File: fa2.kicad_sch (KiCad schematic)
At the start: 7 parts, among them U1 4081, U10 4071, U18 4069, U27 4069, U46 4071, U48 4081, U6 4081

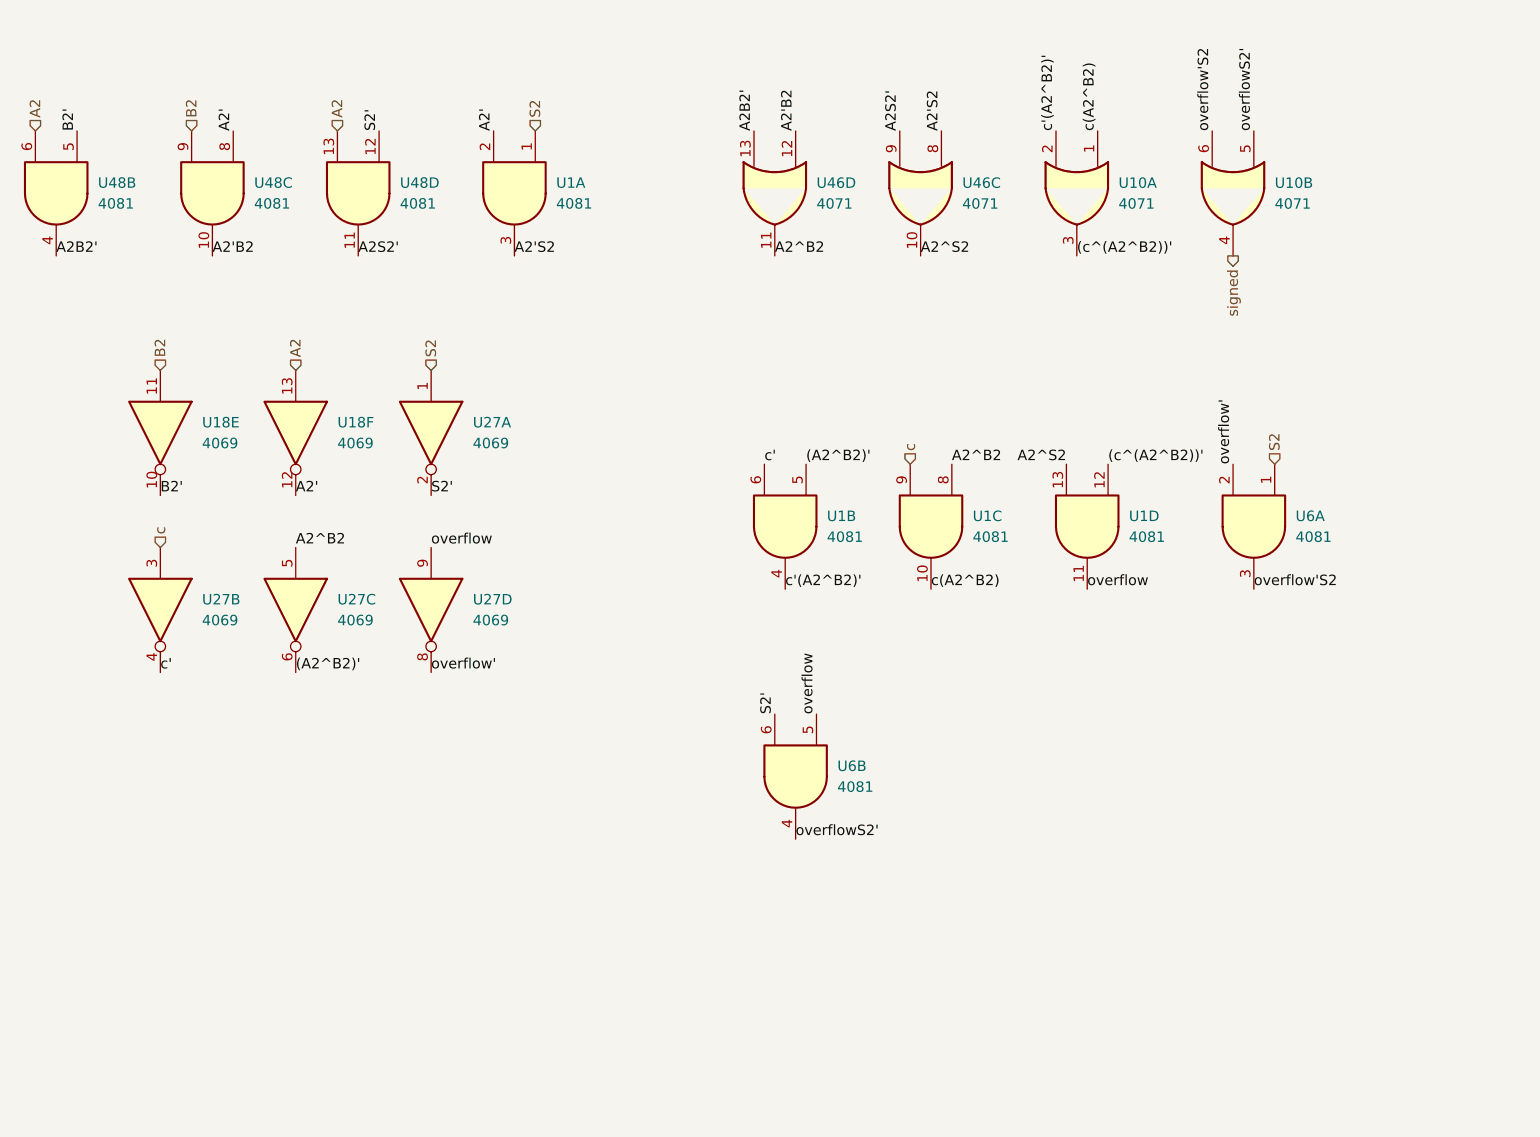
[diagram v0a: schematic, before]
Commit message: Add files via upload
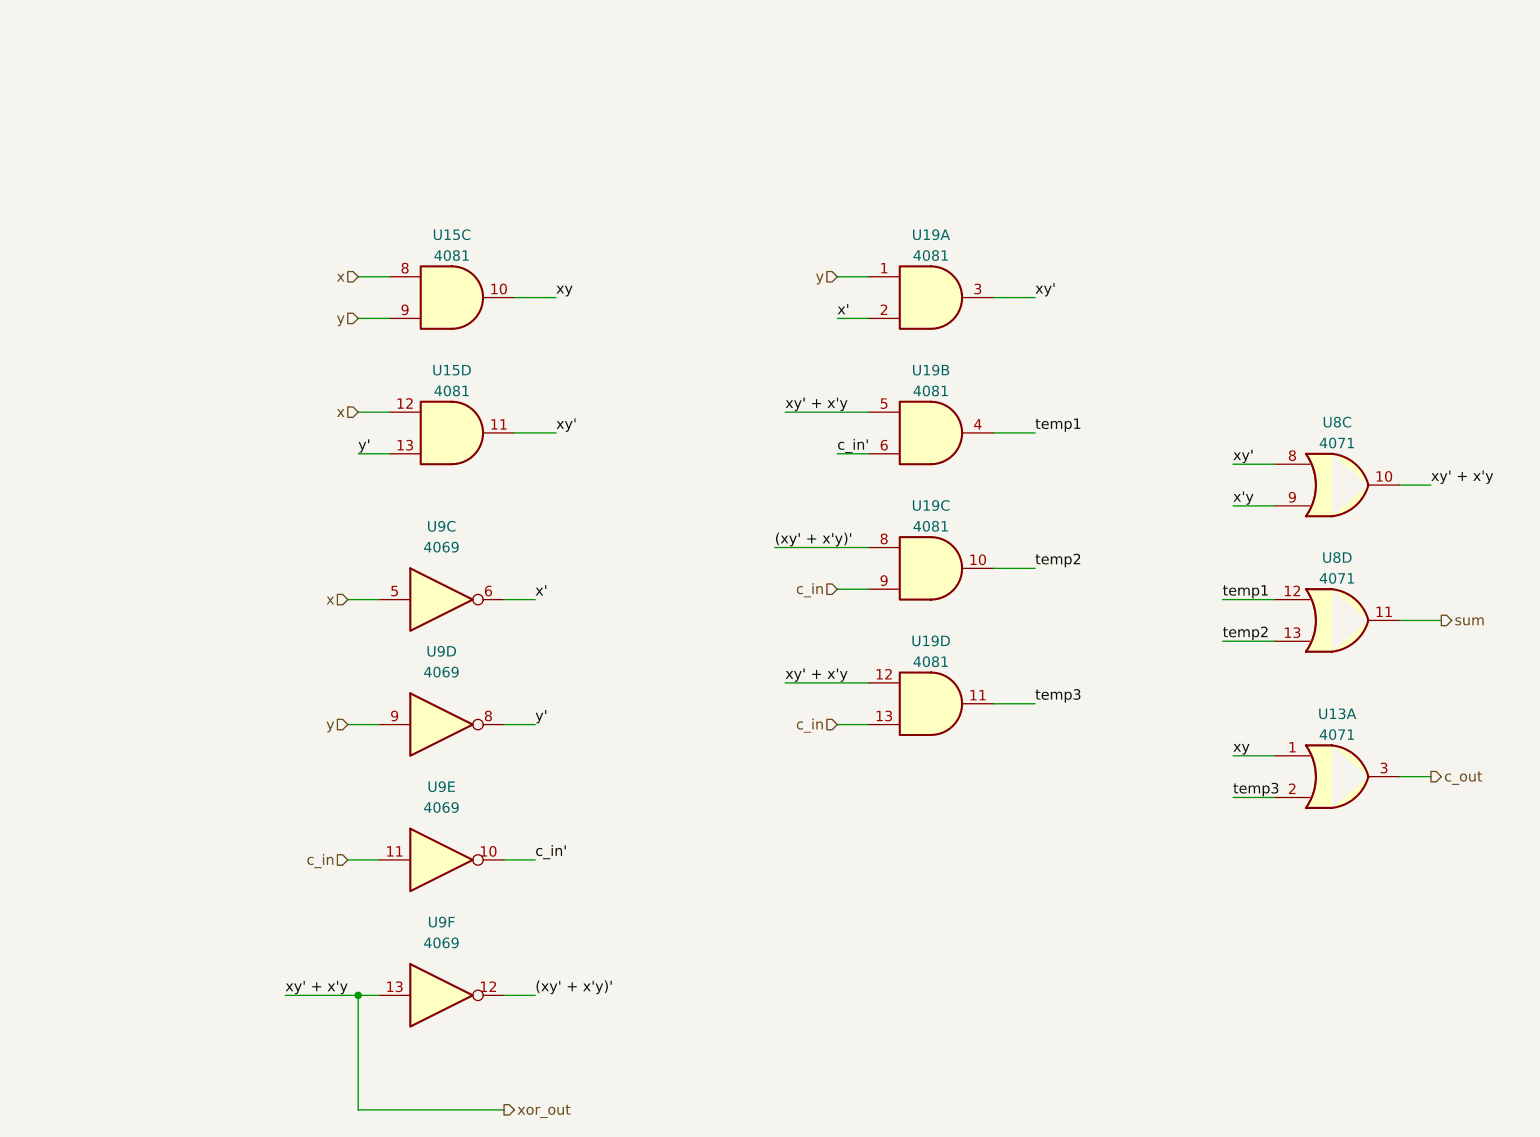
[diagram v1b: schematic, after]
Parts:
- removed U1, U48, U6: 4081, Package_DIP:CERDIP-14_W7.62mm_SideBrazed_LongPads_Socket, symbol 4xxx:4081
- removed U10, U46: 4071, Package_DIP:CERDIP-14_W7.62mm_SideBrazed_LongPads_Socket, symbol 4xxx:4071
- removed U18, U27: 4069, Package_DIP:CERDIP-14_W7.62mm_SideBrazed_LongPads_Socket, symbol 4xxx:4069
- added U13, U8: 4071, Package_DIP:CERDIP-14_W7.62mm_SideBrazed_LongPads_Socket, symbol 4xxx:4071
- added U15, U19: 4081, Package_DIP:CERDIP-14_W7.62mm_SideBrazed_LongPads_Socket, symbol 4xxx:4081
- added U9: 4069, Package_DIP:CERDIP-14_W7.62mm_SideBrazed_LongPads_Socket, symbol 4xxx:4069
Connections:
- new net (xy' + x'y)': U19.8, U9.12
- new net c_in: U19.13, U19.9, U9.11
- new net c_in': U19.6, U9.10
- new net c_out: U13.3
- new net sum: U8.11
- new net temp1: U19.4, U8.12
- new net temp2: U19.10, U8.13
- new net temp3: U13.2, U19.11
- new net x: U15.12, U15.8, U9.5
- new net x': U19.2, U9.6
- new net x'y: U8.9
- new net xor_out: U19.12, U19.5, U8.10, U9.13
- new net xy: U13.1, U15.10
- new net xy': U15.11, U19.3, U8.8
- new net y: U15.9, U19.1, U9.9
- new net y': U15.13, U9.8
